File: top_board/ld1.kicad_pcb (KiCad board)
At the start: 2 copper layers, 62 x 81 mm, 45 parts, among them J1 ENCODER, J2 PROG, J3 MISC, J4 POWER, J5 5V, J6 GND, J7 3V3, J8 GPS+OLED, J9 GND, SW3 KLS7-KL-02-N-0-0, U1 E22-400M30S, U2 ESP32-WROOM-32U

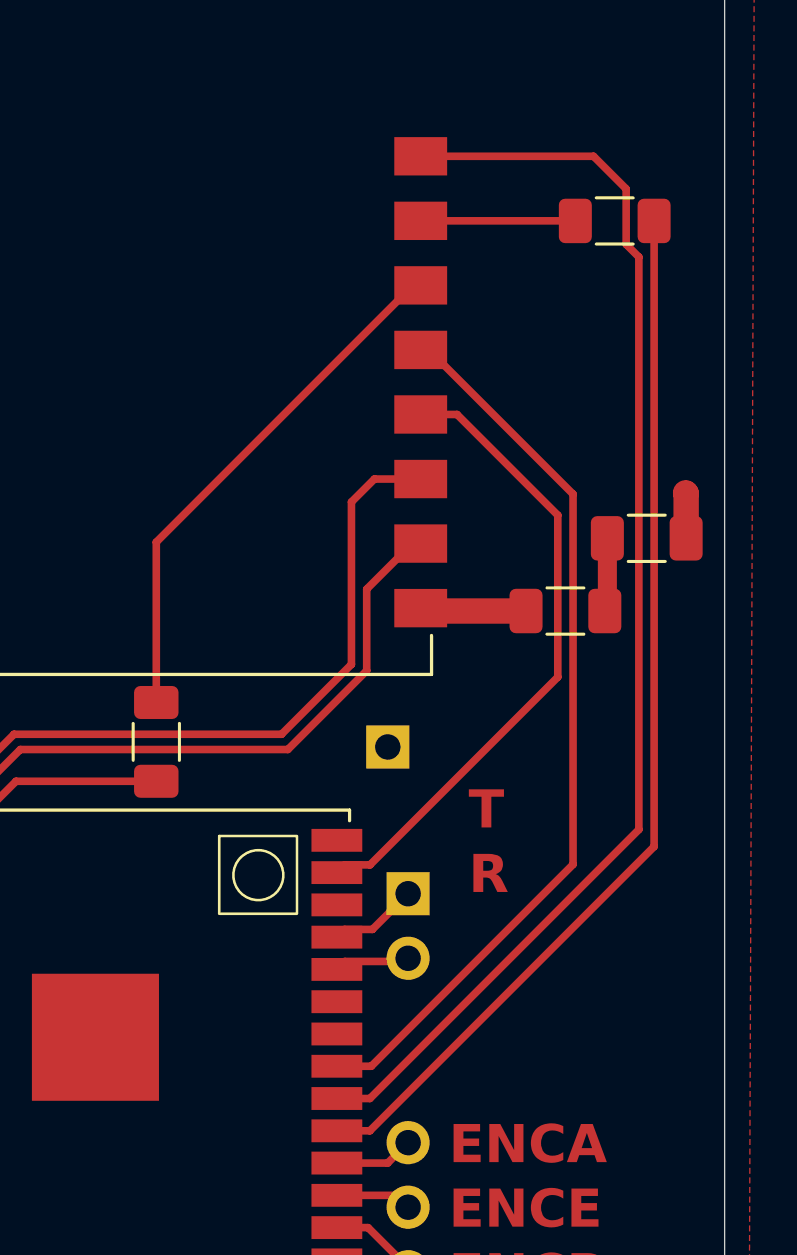
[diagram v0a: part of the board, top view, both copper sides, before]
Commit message: Boards done, composition done
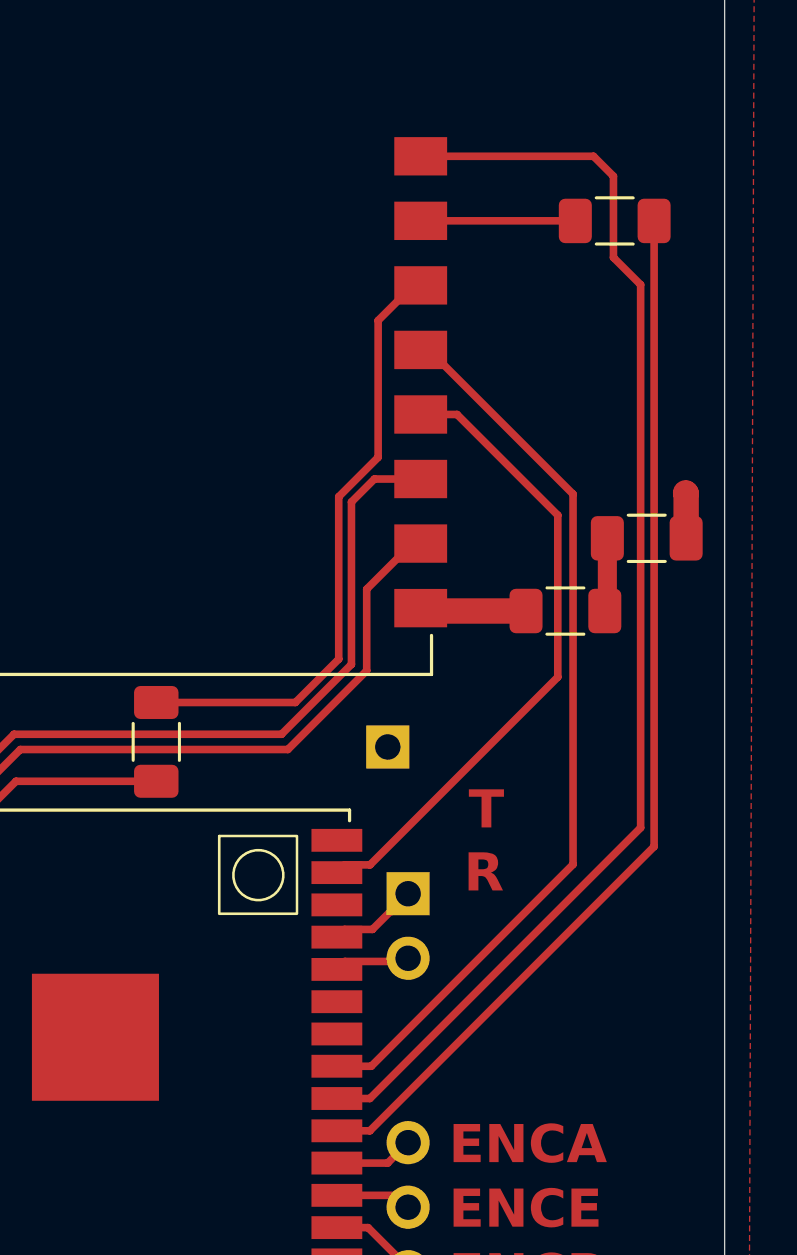
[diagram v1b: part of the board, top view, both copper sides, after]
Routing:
- net MOSI: track 20.9 -> 24.1 mm
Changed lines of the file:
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@@
 	)
 	(gr_text "R"
-		(at 122.38 91.24 0)
+		(at 122.19 91.18 0)
 		(layer "F.Cu")
 		(effects
@@
 	)
 	(segment
-		(start 129.08 88.6)
-		(end 129.08 66.071878)
-		(width 0.3)
-		(layer "F.Cu")
-		(net 9)
-	)
-	(segment
-		(start 118.496 99.184)
-		(end 129.08 88.6)
-		(width 0.3)
-		(layer "F.Cu")
-		(net 9)
-	)
-	(segment
-		(start 129.08 66.071878)
-		(end 128.58 65.571878)
-		(width 0.3)
-		(layer "F.Cu")
-		(net 9)
-	)
-	(segment
-		(start 128.58 65.571878)
-		(end 128.58 63.39)
-		(width 0.3)
-		(layer "F.Cu")
-		(net 9)
-	)
-	(segment
 		(start 117.196 99.184)
 		(end 118.496 99.184)
@@
 	)
 	(segment
-		(start 128.58 63.39)
-		(end 127.296 62.106)
-		(width 0.3)
-		(layer "F.Cu")
-		(net 9)
-	)
-	(segment
 		(start 127.296 62.106)
 		(end 120.4955 62.106)
@@
 	)
 	(segment
+		(start 118.496 99.184)
+		(end 129.15 88.53)
+		(width 0.3)
+		(layer "F.Cu")
+		(net 9)
+	)
+	(segment
+		(start 128.08 62.89)
+		(end 127.296 62.106)
+		(width 0.3)
+		(layer "F.Cu")
+		(net 9)
+	)
+	(segment
+		(start 129.15 67.16)
+		(end 128.08 66.09)
+		(width 0.3)
+		(layer "F.Cu")
+		(net 9)
+	)
+	(segment
+		(start 129.15 88.53)
+		(end 129.15 67.16)
+		(width 0.3)
+		(layer "F.Cu")
+		(net 9)
+	)
+	(segment
+		(start 128.08 66.09)
+		(end 128.08 62.89)
+		(width 0.3)
+		(layer "F.Cu")
+		(net 9)
+	)
+	(segment
 		(start 100.196 97.914)
 		(end 101.716 97.914)
@@
 	)
 	(segment
+		(start 117.27 81.892894)
+		(end 117.27 75.502894)
+		(width 0.3)
+		(layer "F.Cu")
+		(net 11)
+	)
+	(segment
 		(start 110.09 83.6)
-		(end 110.09 77.29)
+		(end 115.562894 83.6)
 		(width 0.3)
 		(layer "F.Cu")
@@
 	)
 	(segment
-		(start 110.09 77.29)
-		(end 120.194 67.186)
+		(start 120.204 67.186)
+		(end 120.4955 67.186)
 		(width 0.3)
 		(layer "F.Cu")
@@
 	)
 	(segment
-		(start 120.194 67.186)
-		(end 120.4955 67.186)
-		(width 0.3)
-		(layer "F.Cu")
+		(start 117.27 75.502894)
+		(end 118.82 73.952894)
+		(width 0.3)
+		(layer "F.Cu")
+		(net 11)
+	)
+	(segment
+		(start 115.562894 83.6)
+		(end 117.27 81.892894)
+		(width 0.3)
+		(layer "F.Cu")
+		(net 11)
+	)
+	(segment
+		(start 118.82 73.952894)
+		(end 118.82 68.57)
+		(width 0.3)
+		(layer "F.Cu")
+		(net 11)
+	)
+	(segment
+		(start 118.82 68.57)
+		(end 120.204 67.186)
+		(width 0.3)
+		(layer "F.Cu")
